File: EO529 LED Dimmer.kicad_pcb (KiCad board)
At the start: 2 copper layers, 77.5 x 58.4 mm, 59 parts, among them J1 VBat, Q1 BC639, Q2 BC639, Q3 BC639, Q4 BC639, U1 NE556, U2 NE556, U3 LM393, U4 LM393

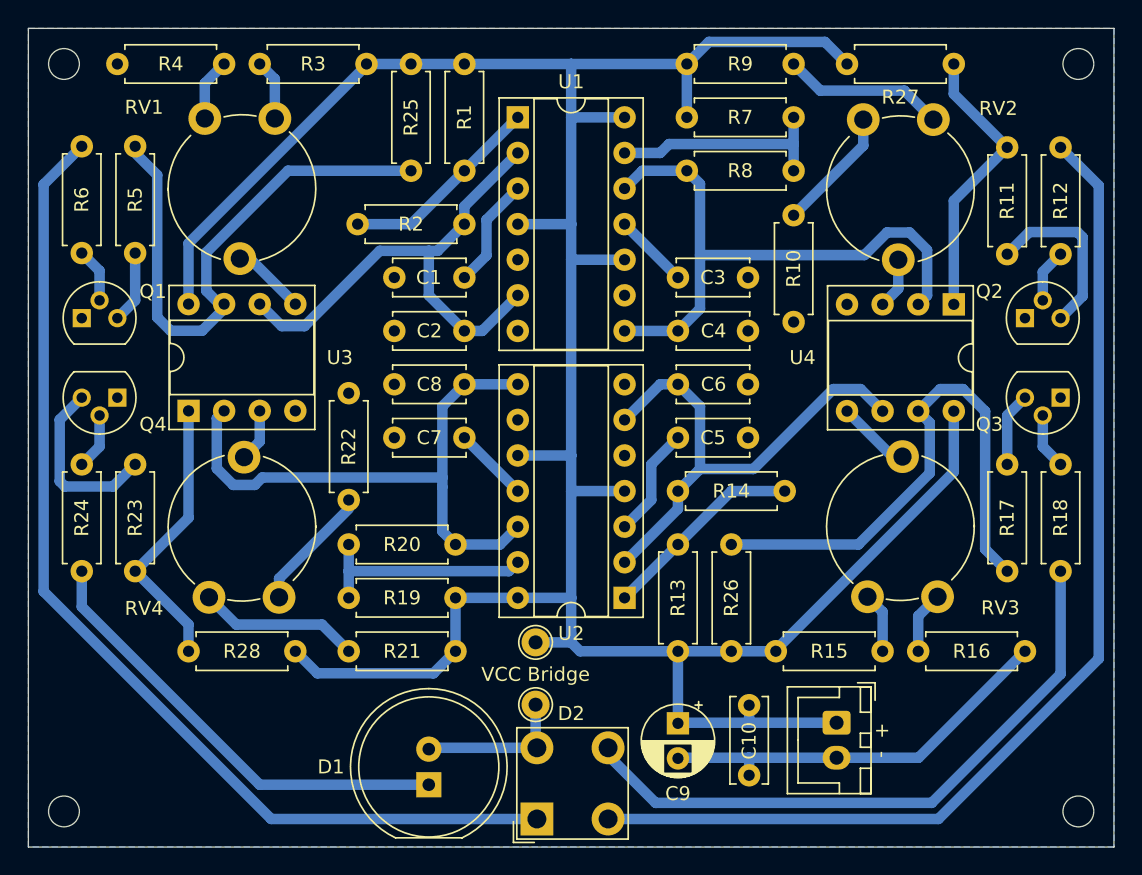
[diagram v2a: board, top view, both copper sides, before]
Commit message: Final revision
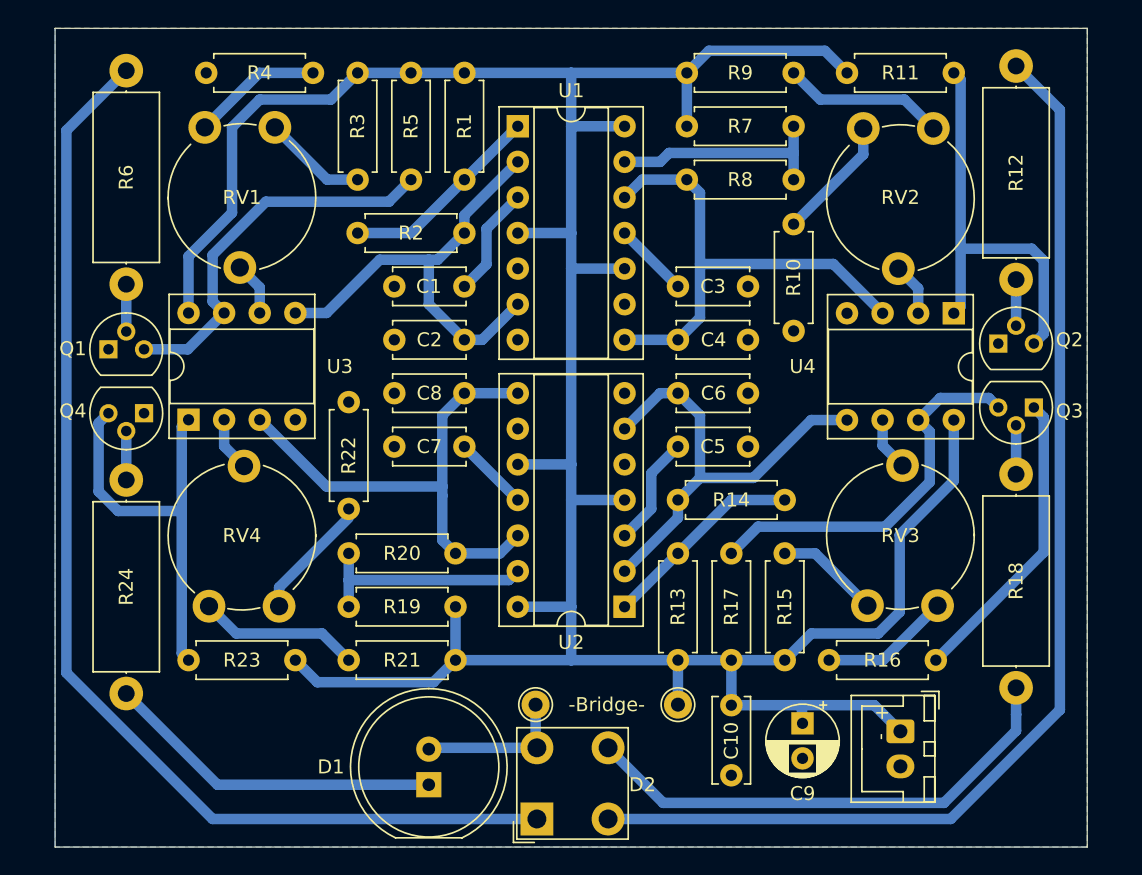
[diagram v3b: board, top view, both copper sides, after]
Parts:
- removed H1, H2, H3, H4: MountingHole, MountingHole:MountingHole_2.2mm_M2
- removed the R11 at (134.6, 85.4)
- removed the R17 at (134.6, 100.4)
- removed the R23 at (72.4, 100.4)
- removed the R5 at (72.4, 85.3)
- R11: renamed from R27; value 1M -> 4.7k
- R12: value 220 -> 180; footprint Resistor_THT:R_Axial_DIN0207_L6.3mm_D2.5mm_P7.62mm_Horizontal -> Resistor_THT:R_Axial_DIN0414_L11.9mm_D4.5mm_P15.24mm_Horizontal
- R17: renamed from R26; value 1M -> 4.7k
- R18, R6: footprint Resistor_THT:R_Axial_DIN0207_L6.3mm_D2.5mm_P7.62mm_Horizontal -> Resistor_THT:R_Axial_DIN0414_L11.9mm_D4.5mm_P15.24mm_Horizontal
- R23: renamed from R28; value 1M -> 4.7k
- R24: value 180 -> 220; footprint Resistor_THT:R_Axial_DIN0207_L6.3mm_D2.5mm_P7.62mm_Horizontal -> Resistor_THT:R_Axial_DIN0414_L11.9mm_D4.5mm_P15.24mm_Horizontal
- R5: renamed from R25; value 1M -> 4.7k
- moved TP2 11.1 mm to (111.1, 117.5)
- moved C9 8.89 mm to (120.0, 118.9)
- moved R16 6.40 mm to (121.9, 114.4)
- moved R4 6.37 mm to (85.1, 72.5)
- moved J1 4.60 mm to (127.0, 119.4)
- moved R6 3.88 mm to (71.8, 87.5)
- moved R12 3.66 mm to (135.3, 87.2)
- moved R24 3.36 mm to (71.8, 101.5)
- moved R18 3.25 mm to (135.3, 101.1)
- moved Q1 2.93 mm to (70.5, 92.2)
- moved Q2 2.63 mm to (134.0, 91.8)
- moved Q4 2.21 mm to (73.0, 96.7)
- moved Q3 2.03 mm to (136.5, 96.3)
- moved C10 1.27 mm to (114.9, 117.6)
- moved R3 0.90 mm to (88.3, 72.5), turned to -90 degrees
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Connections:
- R11 pad 1: Net-(R11-Pad2) -> Net-(Q2-Pad3)
- R17 pad 1: Net-(U4-Pad7) -> Net-(Q3-Pad3)
- R23 pad 1: Net-(R23-Pad2) -> Net-(Q4-Pad3)
- R5 pad 1: Net-(U3-Pad7) -> Net-(Q1-Pad3)
- U3 pad 1: Net-(R23-Pad2) -> Net-(Q4-Pad3)
- U3 pad 2: Net-(C8-Pad1) -> Net-(RV4-Pad2)
- U3 pad 3: Net-(RV4-Pad2) -> Net-(C8-Pad1)
- U3 pad 5: Net-(RV1-Pad2) -> Net-(C2-Pad1)
- U3 pad 6: Net-(C2-Pad1) -> Net-(RV1-Pad2)
- U3 pad 7: Net-(U3-Pad7) -> Net-(Q1-Pad3)
- U4 pad 1: Net-(R11-Pad2) -> Net-(Q2-Pad3)
- U4 pad 2: Net-(C4-Pad1) -> Net-(RV2-Pad2)
- U4 pad 3: Net-(RV2-Pad2) -> Net-(C4-Pad1)
- U4 pad 5: Net-(RV3-Pad2) -> Net-(C6-Pad1)
- U4 pad 6: Net-(C6-Pad1) -> Net-(RV3-Pad2)
- U4 pad 7: Net-(U4-Pad7) -> Net-(Q3-Pad3)
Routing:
- net Net-(U3-Pad7): track 39.8 -> 0.00 mm
- net Net-(U4-Pad7): track 39.2 -> 0.00 mm
- net Net-(Q1-Pad3): track 5.17 -> 27.7 mm
- net Net-(Q3-Pad3): track 5.29 -> 27.7 mm
- net Net-(R11-Pad2): track 20.3 -> 0.00 mm
- net Net-(R23-Pad2): track 20.0 -> 0.00 mm
- net Net-(Q2-Pad3): track 12.6 -> 30.1 mm
- net Net-(Q4-Pad3): track 12.8 -> 29.9 mm
- net VCC: track 204.5 -> 215.4 mm
- net Blue: track 45.4 -> 35.9 mm
- net Net-(D1-Pad1): track 32.6 -> 24.3 mm
- net Red: track 74.8 -> 82.6 mm
- net GND: track 29.2 -> 21.5 mm
- net Net-(C4-Pad1): track 42.8 -> 35.7 mm
- net Net-(C8-Pad1): track 42.4 -> 36.3 mm
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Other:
- board size 77.5 x 58.4 mm -> 73.7 x 58.4 mm
- board text added: "-Bridge-"
- board text removed: "VCC Bridge"
